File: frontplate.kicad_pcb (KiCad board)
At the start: 2 copper layers, 200 x 105 mm, 5 parts

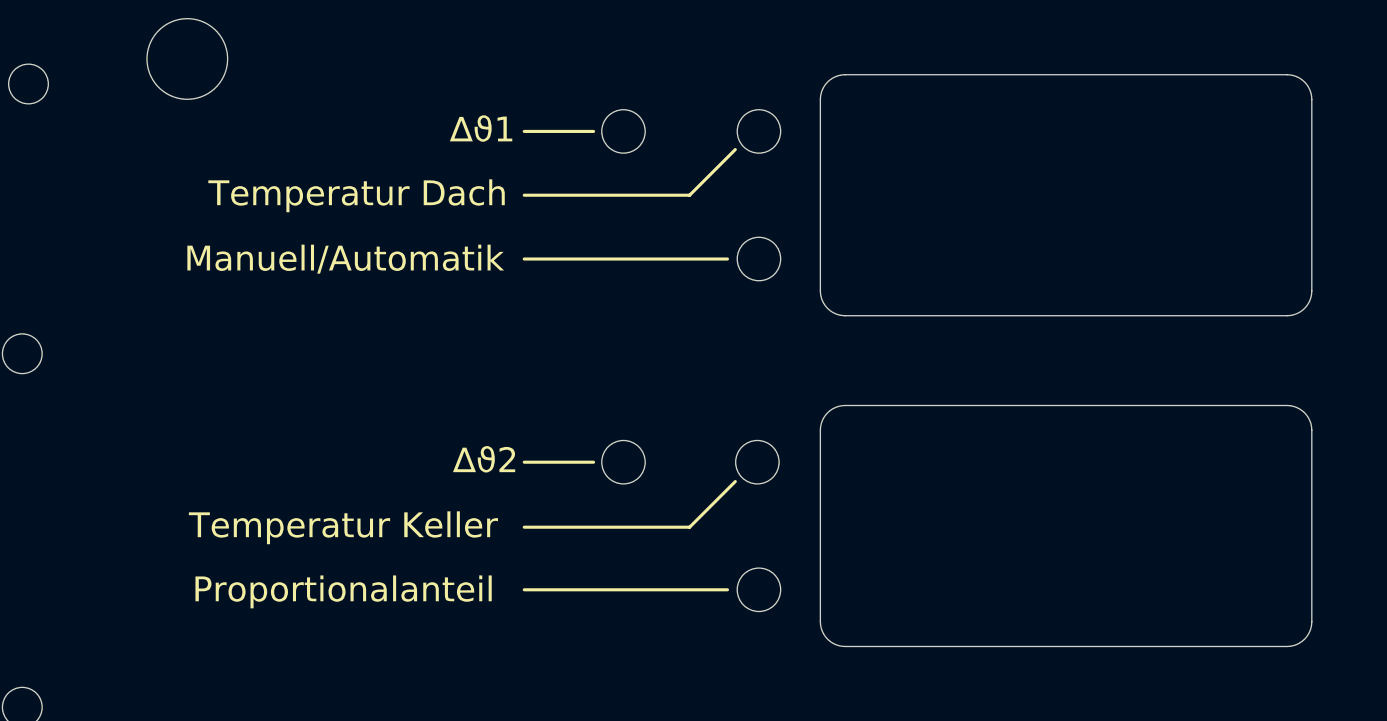
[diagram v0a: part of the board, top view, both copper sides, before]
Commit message: Rev.B -> Rev.C
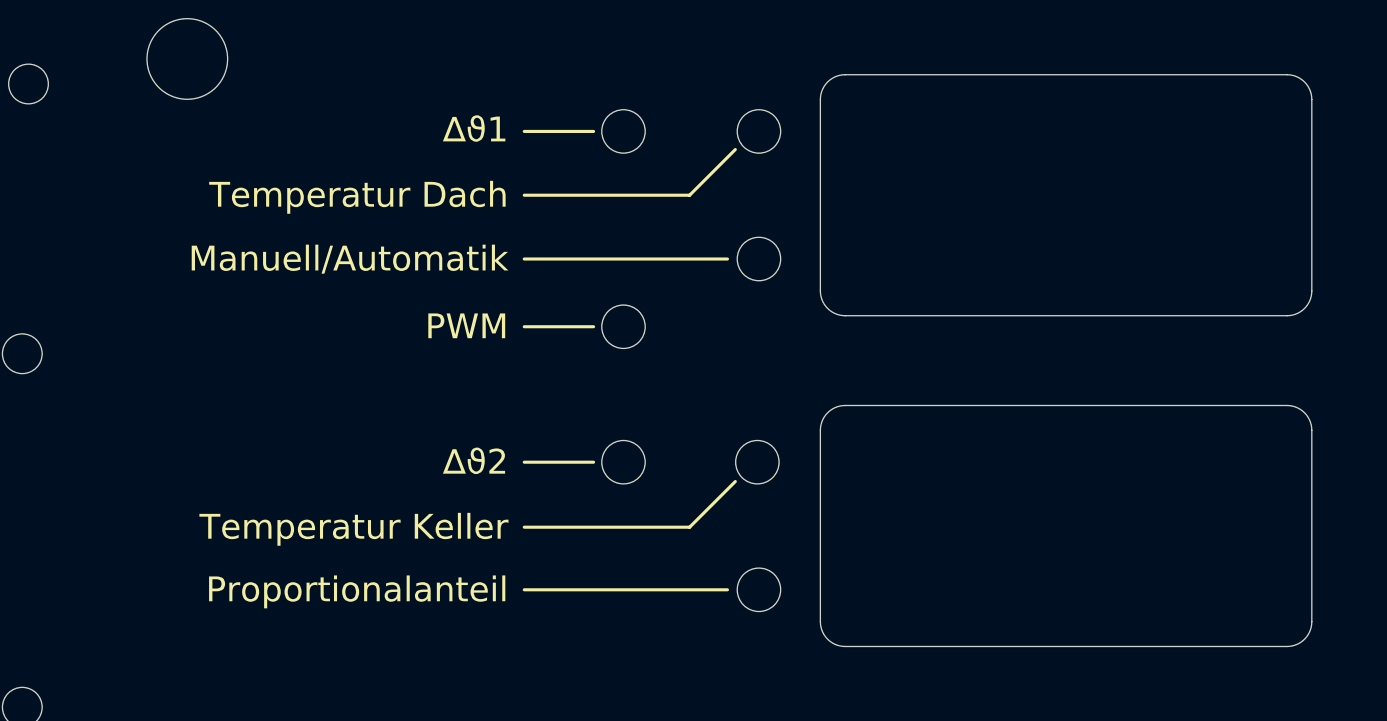
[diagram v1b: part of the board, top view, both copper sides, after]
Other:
- outline, holes or cut-outs redrawn
- net class Default removed
- board text added: "PWM"
